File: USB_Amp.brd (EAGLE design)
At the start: 88 x 60 mm, 202 parts, among them CON1 AUDIO_IN, CON2 PROG, CON3 PWR IN, CON4 USB-C-2OZ, CON5 SWD, IC1 ISO7762, IC10 74LVC1G79, IC11 1.8V, IC12 AK1110, IC13 STM32G030F, IC14 CH221, IC15 7808, IC16 TAR5SB33, IC2 3.3V, IC3 PIC32MZEF, IC4 TAR5SB33, IC5 SSM3582, IC6 3G04, IC7 TL431, IC8 74LVC1G79, IC9 74LVC1G79, Q1 PNP, Q2 PNP, Q3 PNP, Q4 NPN, Q5 NPN, X1 12MHz, X2 22.5792MHz, X3 24.576MHz

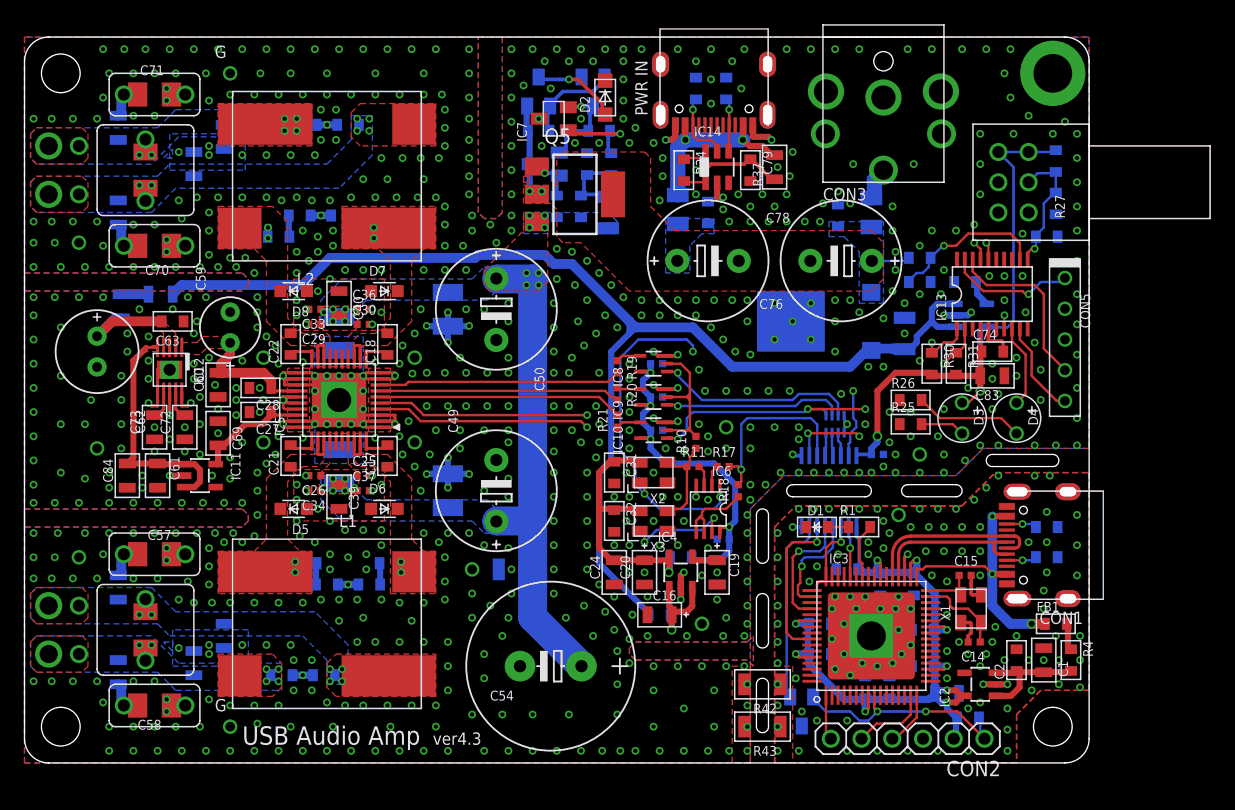
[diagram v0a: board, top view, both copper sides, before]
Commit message: v6
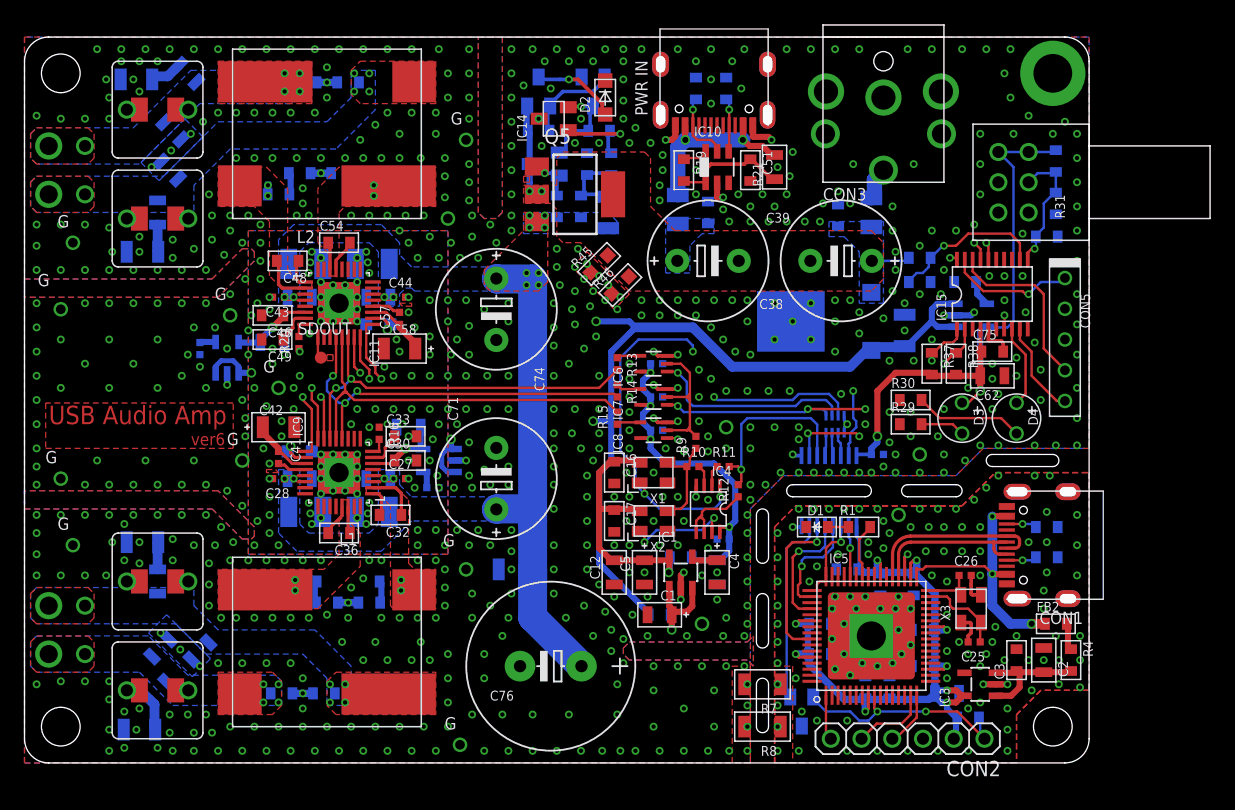
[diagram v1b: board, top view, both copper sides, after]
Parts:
- removed D5, D6, D7, D8: SBD, my_rcl:SOD323
- removed FB6: FB, my_rcl:3216-FB
- added C89: 10n, my_rcl:3216
- added C90, C91: 0.1u, my_rcl:1005
- added IC17: 3.3V, my_ic:SOT23-5
- added R44: 1.5k, my_rcl:1608
- added R45, R46: THJ, my_rcl:1608-W
- added TP23: SDOUT, my_connector:TESTPAD-SMALL
- added TP24: G, my_connector:TESTPIN
- C1, C5: device my_rcl:2012 -> my_rcl:2012-POL
- C12: value 0.1u -> 2.2u; device my_rcl:1608C -> my_rcl:2012
- C13: value 1u -> 0.1u
- C14, C15: value 10p -> 0.1u; device my_rcl:1005 -> my_rcl:1608C
- C16: value 10u -> 0.1u; device my_rcl:2012-POL -> my_rcl:1608C
- C17, C18: value 0.22u -> 0.1u
- C19: value 2.2u -> 0.1u; device my_rcl:2012-POL -> my_rcl:1608C
- C2: value 1u -> 10u; device my_rcl:1608C -> my_rcl:2012
- C20: value 10u -> 0.1u; device my_rcl:2012-POL -> my_rcl:1005
- C21: value 0.22u -> 1u
- C22: value 0.22u -> 0.1u; device my_rcl:1608C -> my_rcl:1005
- C23: value 10u -> 1u; device my_rcl:2012 -> my_rcl:1005
- C24: value 2.2u -> 0.1u; device my_rcl:2012 -> my_rcl:1005
- C25, C26: value 10n -> 10p
- C27, C28, C7: device my_rcl:1608C -> my_rcl:1005
- C29: value 10n -> 1u; device my_rcl:1005 -> my_rcl:2012
- C3: value 0.1u -> 1u
- C30: value 10n -> 1u; device my_rcl:1005 -> my_rcl:1608C
- C31: value 0.1u -> 1u; device my_rcl:1608C -> my_rcl:2012
- C32: value 0.1u -> 0.47u
- C33: value 0.1u -> 1u; device my_rcl:1005 -> my_rcl:1608C
- C34, C35: value 0.1u -> 10u; device my_rcl:1005 -> my_rcl:3225
- C36: value 0.1u -> 0.47u; device my_rcl:1005 -> my_rcl:1608C
- C37: device my_rcl:1005 -> my_rcl:1608C
- C38: value 0.1u -> 25V 1000u; device my_rcl:1005 -> my_rcl:E5-10
- C39: value 1u -> 25V 1000u; device my_rcl:2012 -> my_rcl:E5-10
- C4: value 0.1u -> 2.2u; device my_rcl:1005 -> my_rcl:2012-POL
- C40: device my_rcl:2012 -> my_rcl:1608-W
- C42: value DNP -> 1u; device my_rcl:1608C -> my_rcl:3216-POL
- C43, C44: value 10u -> 0.1u; device my_rcl:3225 -> my_rcl:1005
- C45: value 0.1u -> 1u; device my_rcl:1005 -> my_rcl:2012
- C46: value 10u -> 1u; device my_rcl:3225 -> my_rcl:1608C
- C47: value 10u -> 1u; device my_rcl:3225 -> my_rcl:2012
- C48: value 4.7u -> 0.47u; device my_rcl:3216 -> my_rcl:1608C
- C49: value 16V 680u -> 1u; device my_rcl:E5-10 -> my_rcl:1608C
- C50: value 16V 680u -> 10u; device my_rcl:E5-10 -> my_rcl:3225
- C51: value 100p -> 1u
- C52: value 0.22u -> 10u; device my_rcl:C050W -> my_rcl:3225
- C53: value 100p -> 0.1u
- C54: value 16V 2200u -> 0.47u; device my_rcl:E5-13 -> my_rcl:1608C
- C55: value 1n -> 10u; device my_rcl:2012 -> my_rcl:3216
- C56: value 1n -> 1u; device my_rcl:2012 -> my_rcl:1608-W
- C57: value 10n -> 0.1u; device my_rcl:C050W2 -> my_rcl:1005
- C58: value 10n -> 1u; device my_rcl:C050W2 -> my_rcl:3216-POL
- C59: value 47u -> 0.1u; device my_rcl:E2.5-5 -> my_rcl:1608C
- C60: value 10u -> 100p; device my_rcl:2012 -> my_rcl:1608C
- C61: value 4.7u -> 100p; device my_rcl:2012 -> my_rcl:1608C
- C62: value 100u -> 22u; device my_rcl:E2.5-6.5 -> my_rcl:2012
- C63: value 0.1u -> DNP
- C65: value 0.22u -> 100p; device my_rcl:C050W -> my_rcl:1608C
- C66: value 100p -> 0.47u; device my_rcl:1608C -> my_rcl:C050W
- C67: value 1n -> 0.47u; device my_rcl:2012 -> my_rcl:C050W
- C68: value 1n -> 4.7u; device my_rcl:2012 -> my_rcl:3216
- C69: value 10u -> 1n
- C70: value 10n -> 1n; device my_rcl:C050W2 -> my_rcl:2012
- C71: value 10n -> 16V 680u; device my_rcl:C050W2 -> my_rcl:E5-10
- C72, C73: value 10u -> 10n; device my_rcl:2012 -> my_rcl:3216
- C74: value 0.1u -> 16V 680u; device my_rcl:1608C -> my_rcl:E5-10
- C76: value 25V 1000u -> 16V 2200u; device my_rcl:E5-10 -> my_rcl:E5-13
- C78: value 25V 1000u -> 100p; device my_rcl:E5-10 -> my_rcl:1608C
- C79: value 1u -> 100p
- C8, C9: value 0.1u -> 10u; device my_rcl:1608C -> my_rcl:2012
- C80: value 0.1u -> 100p
- C81: value 10u -> 100p; device my_rcl:3216 -> my_rcl:1608C
- C82: value 0.1u -> 0.47u; device my_rcl:1608C -> my_rcl:C050W
- C83: value 22u -> 0.47u; device my_rcl:2012 -> my_rcl:C050W
- C84: value 4.7u -> 10u
- C85: value 100p -> 10u; device my_rcl:1608C -> my_rcl:2012
- C86, C87: value 100p -> 1n; device my_rcl:1608C -> my_rcl:2012
- C88: value 100p -> 10n; device my_rcl:1608C -> my_rcl:3216
- FB4: device my_rcl:2012-R -> my_rcl:3216-FB
- IC1: value ISO7762 -> TAR5SB33; device my_ic:TSSOP16 -> my_ic:SOT23-5
- IC10: value 74LVC1G79 -> CH221; device my_ic:TSSOP5 -> my_ic:SOT23-6
- IC11: value 1.8V -> TAS5827; device my_ic:SOT23-5 -> my_ic:QFN32-TAS
- IC12: value AK1110 -> 7805; device my_ic:PLP10 -> my_ic:DPAK
- IC13: value STM32G030F -> TAR5SB33; device my_ic:TSSOP20 -> my_ic:SOT23-5
- IC14: value CH221 -> TL431; device my_ic:SOT23-6 -> my_ic:SC59
- IC15: value 7808 -> STM32G030F; device my_ic:DPAK -> my_ic:TSSOP20
- IC16: value TAR5SB33 -> 3.3V
- IC2: value 3.3V -> ISO7762; device my_ic:SOT23-5 -> my_ic:TSSOP16
- IC3: value PIC32MZEF -> 3.3V; device my_ic:QFN64HT -> my_ic:SOT23-5
- IC4: value TAR5SB33 -> 3G04; device my_ic:SOT23-5 -> my_ic:SSOP8-P-0.65
- IC5: value SSM3582 -> PIC32MZEF; device my_ic:QFN40HT -> my_ic:QFN64HT
- IC6: value 3G04 -> 74LVC1G79; device my_ic:SSOP8-P-0.65 -> my_ic:TSSOP5
- IC7: value TL431 -> 74LVC1G79; device my_ic:SC59 -> my_ic:TSSOP5
- IC9: value 74LVC1G79 -> TAS5827; device my_ic:TSSOP5 -> my_ic:QFN32-TAS
- R11: value 51 -> MCLK
- R12: value 39.2k -> MCLKB; device my_rcl:1608 -> my_rcl:1005
- R13: value 10k -> DATA; device my_rcl:1608 -> my_rcl:1005
- R14: value 1k -> LRCLK; device my_rcl:3216 -> my_rcl:1005
- R15: value 51 -> SCK; device my_rcl:2012 -> my_rcl:1005
- R16: value 51 -> 0; device my_rcl:2012 -> my_rcl:1005
- R17: value MCLK -> 5.1k; device my_rcl:1005 -> my_rcl:1608
- R18: value MCLKB -> 5.1k; device my_rcl:1005 -> my_rcl:1608
- R19: value SCK -> 200k; device my_rcl:1005 -> my_rcl:1608
- R20: value DATA -> 1k
- R21: value LRCLK -> 1k; device my_rcl:1005 -> my_rcl:2012
- R22: value 2.2 -> 100; device my_rcl:2012-R -> my_rcl:1608
- R23, R24: value 51 -> 10; device my_rcl:2012 -> my_rcl:1608
- R25, R26: value 3.3k -> 1k
- R27: value 50k -> 40.2k; device my_rcl:RK0972 -> my_rcl:1608
- R28: value DNP -> 10k
- R29: value 100k -> 3.3k
- R30: value 10k -> 3.3k
- R31: value 10k -> 50k; device my_rcl:1608 -> my_rcl:RK0972
- R32, R33: value 5.1k -> 5.1; device my_rcl:1608 -> my_rcl:2012
- R34: value 100k -> 1k; device my_rcl:1608 -> my_rcl:3216
- R35: value 10k -> DNP
- R36: value 1.5k -> 100k
- R37: value 1k -> 10k; device my_rcl:2012 -> my_rcl:1608
- R38: value 10 -> 10k
- R41: value 10 -> 5.1; device my_rcl:1608 -> my_rcl:2012
- R42: value THJ -> 5.1; device my_rcl:3216-2 -> my_rcl:2012
- R43: value THJ -> 10k; device my_rcl:3216-2 -> my_rcl:1608
- R7: value 100 -> THJ; device my_rcl:1608 -> my_rcl:3216-2
- R8: value 1k -> THJ; device my_rcl:1608 -> my_rcl:3216-2
- R9: value 1k -> 51; device my_rcl:1608 -> my_rcl:1005
- TP19: value L_P -> L_N
- TP22, TP4: value R_N -> R_P
- TP3: value R_P -> R_N
- X1: value 12MHz -> 22.5792MHz; device my_rcl:KC3225-CRYSTAL -> my_rcl:KC3225
- X2: value 22.5792MHz -> 24.576MHz
- X3: value 24.576MHz -> 12MHz; device my_rcl:KC3225 -> my_rcl:KC3225-CRYSTAL
- moved C62 74.0 mm to (80.0, 32.0), turned to 0 degrees
- moved C83 72.4 mm to (11.0, 54.0), turned to 180 degrees
- moved R42 69.3 mm to (13.5, 57.0), flipped to the bottom, turned to 225 degrees
- moved C82 67.0 mm to (11.0, 45.0), flipped to the top
- moved R33 66.7 mm to (11.0, 6.00), turned to 135 degrees
- moved R32 62.2 mm to (11.0, 15.0)
- moved C55 61.7 mm to (72.8, 35.8)
- moved C59 60.9 mm to (77.8, 39.8), flipped to the bottom, turned to 0 degrees
- moved FB4 59.1 mm to (70.0, 45.5), turned to 270 degrees
- moved IC12 58.1 mm to (70.0, 36.5), flipped to the bottom, turned to 270 degrees
- moved R38 56.2 mm to (77.0, 33.0), flipped to the top, turned to 270 degrees
- moved C51 54.6 mm to (60.0, 49.0), flipped to the top, turned to 270 degrees
- moved C26 54.4 mm to (77.8, 15.5), turned to 0 degrees
- moved C81 53.7 mm to (23.2, 56.2), turned to 180 degrees
- moved C21 53.1 mm to (71.5, 6.25), flipped to the bottom
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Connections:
- removed net +8V: C81.1, FB2.1, FB4.1, IC15.3, IC16.1, IC16.3
- removed net AMP_+5V: C61.1, C84.1, IC11.1, IC11.3, IC12.5
- removed net AMP_AVDD: C28.1, C59.+, C60.1, IC12.1, IC5.24
- removed net AMP_DVDD: C27.1, C69.1, IC11.5, IC5.28
- new net +5V: C55.1, FB1.1, IC12.3, IC13.1, IC13.3, IC16.1, IC16.3, IC17.1, IC17.3
- new net AMP_AVDD_L: C41.1, C42.1, IC9.19
- new net AMP_AVDD_R: C57.1, C58.1, IC11.19
- new net AMP_DVDD_L: C30.1, C84.1, IC16.5, IC9.6
- new net AMP_DVDD_R: C46.1, C85.1, IC11.6, IC17.5
- new net AMP_EN: IC11.17, IC15.20, IC9.17
- new net AMP_IO0: IC11.9, TP23.1
- new net N$47: IC11.8, R20.2
- new net N$48: C33.1, IC9.7
- new net N$49: C90.1, IC16.4
- new net N$50: C91.1, IC17.4
- net +12V: now also C27.1, C28.1, C31.1, C35.1, C45.1, C50.1, C52.1, C68.1, C71.+, C74.+, C76.+, IC11.21, IC11.22, IC11.3, IC11.4, IC9.21, IC9.22, IC9.3, IC9.4, R25.2, R27.2, R34.2; no longer C25.1, C26.1, C30.1, C33.1, C36.1, C37.1, C39.1, C40.1, C46.1, C48.1, C49.+, C50.+, C54.+, IC5.14, IC5.15, IC5.16, IC5.17, IC5.34, IC5.35, IC5.36, IC5.37, R12.2, R14.2, R8.2
- net +3V3: now also C62.1, C7.1, C75.1, IC13.5, IC15.4, IC2.16, R31.3, R31.6, R35.2, R37.2, R38.2; no longer C4.1, C74.1, C83.1, IC1.16, IC13.4, IC16.5, R27.3, R27.6, R28.2, R30.2, R31.2
- net +3V3A: now also C20.1, C22.1, C24.1, C8.1, IC4.8, IC6.5, IC7.5; no longer C35.1, C38.1, C41.1, C45.1, IC10.5, IC6.8, IC9.5
- net +3V3D: now also C14.1, C15.1, C18.1, C19.1, C21.1, IC2.1, IC3.5, IC5.19, IC5.26, IC5.34, IC5.39, IC5.54, IC5.60, IC5.8; no longer C12.1, C3.1, C5.1, C7.1, C8.1, IC1.1, IC2.5, IC3.19, IC3.26, IC3.34, IC3.39, IC3.54, IC3.60, IC3.8
- net AMP_OUTN_L: now also C36.1, IC9.30, R24.2; no longer C21.1, D5.2, IC5.32, IC5.33, R38.2
- net AMP_OUTN_R: now also C54.1, IC11.30, L2.1, R39.2; no longer C22.2, D8.2, IC5.18, IC5.19, L2.4, R40.2
- net AMP_OUTP_L: now also C32.1, IC9.2, R23.2; no longer C17.1, D6.2, IC5.38, IC5.39, R39.2
- net AMP_OUTP_R: now also C48.2, IC11.2, L2.4, R40.2; no longer C18.2, D7.2, IC5.12, IC5.13, L2.1, R41.2
- net DGND: now also C18.2, C19.2, C21.2, C25.2, C26.2, IC2.8, IC3.2, IC5.20, IC5.25, IC5.35, IC5.40, IC5.55, IC5.59, IC5.7, IC5.HT, IC5.HT2, R7.1, R8.1, X3.2, X3.4; no longer C1.2, C12.2, C5.2, C7.2, C8.2, IC1.8, IC2.2, IC3.20, IC3.25, IC3.35, IC3.40, IC3.55, IC3.59, IC3.7, IC3.HT, IC3.HT2, R42.1, R43.1, X1.2, X1.4
- net EN_441K: now also IC15.17, IC2.15, IC4.1, X1.1; no longer IC1.15, IC13.17, IC6.1, X2.1
- net EN_48K: now also IC4.7, X2.1; no longer IC6.7, X3.1
- net GND: now also C1.2, C12.2, C17.2, C22.2, C38.-, C39.-, C42.2, C49.2, C5.2, C50.2, C51.2, C52.2, C55.2, C57.2, C59.2, C62.2, C65.2, C66.1, C66.3, C67.2, C67.4, C69.1, C7.2, C70.2, C71.-, C72.1, C74.-, C78.2, C8.2, C80.1, C82.1, C82.3, C83.4, C86.1, C88.1, C89.2, C90.2, C91.2, IC1.2, IC10.2, IC11.20, IC11.25, IC11.26, IC11.31, IC11.32, IC11.5, IC11.HT, IC11.HT2, IC12.2, IC13.2, IC14.3, IC15.5, IC17.2, IC2.9, IC4.4, IC6.3, IC9.20, IC9.25, IC9.26, IC9.31, IC9.32, IC9.5, IC9.HT, IC9.HT2, R16.1, R17.2, R18.2, R20.1, R28.1, R30.1, R31.1, R31.4, R34.1, R36.1, R44.2, R45.1, R46.1, R7.2, R8.2, TP24.1, X1.2; no longer C19.2, C25.2, C26.2, C32.2, C36.2, C38.2, C39.2, C49.-, C50.-, C51.1, C54.-, C55.1, C57.1, C57.3, C58.4, C59.-, C62.-, C63.2, C66.2, C67.1, C68.2, C69.2, C70.1, C70.3, C71.2, C71.4, C72.2, C74.2, C78.-, C80.2, C82.2, C86.2, C88.2, D5.1, D6.1, D7.1, D8.1, IC1.9, IC10.3, IC11.2, IC12.10, IC12.6, IC12.8, IC12.HT, IC12.HT2, IC13.5, IC14.2, IC15.2, IC4.2, IC5.1, IC5.10, IC5.2, IC5.21, IC5.22, IC5.23, IC5.25, IC5.26, IC5.27, IC5.29, IC5.3, IC5.30, IC5.9, IC5.HT, IC5.HT2, IC6.4, IC9.3, R13.1, R14.1, R25.1, R26.1, R27.1, R27.4, R32.2, R33.2, R36.2, R42.2, R43.2, X3.2
- net I2C_SCL: now also IC11.16, IC15.1, IC9.16, R37.1; no longer IC13.1, IC5.4, R30.1
- net I2C_SDA: now also IC11.15, IC15.2, IC9.15, R38.1; no longer IC13.2, IC5.5, R31.1
- net I2S_DATA: now also IC6.1; no longer IC9.1
- net I2S_DATA_BUF: now also IC11.14, IC9.14, R13.2; no longer IC5.7, R20.2
- net I2S_LRCLK: now also IC15.7, IC7.1; no longer IC10.1, IC13.7
- net I2S_LRCLK_BUF: now also IC11.12, IC9.12, R14.2; no longer IC5.6, R21.2
- net I2S_MCLK: now also IC6.2, IC7.2, R9.2; no longer IC10.2, IC9.2, R10.2
- net I2S_MCLK2: now also IC4.3, R10.2; no longer IC6.3, R11.2
- net I2S_MCLK_BUF: now also IC2.11, R11.2, R12.2; no longer IC1.11, R17.2, R18.2
- net I2S_SCK_BUF: now also IC11.13, IC9.13, R15.2; no longer IC5.8, R19.2
- net LED0: now also IC15.8; no longer IC13.8
- net LED1: now also IC5.42; no longer IC3.42
- net MCLK_OSC: now also R9.1, X1.3; no longer R11.1, X3.3
- net MCLR: now also IC5.9; no longer IC3.9
- net N$10: now also IC6.4, R13.1; no longer IC8.4, R19.1
- net N$11: now also IC7.4, R14.1; no longer IC9.4, R20.1
- net N$12: now also C54.2, IC11.29; no longer C21.2, IC5.31
- net N$13: now also C32.2, IC9.1; no longer C17.2, IC5.40
- net N$14: now also IC8.4, R15.1; no longer IC10.4, R21.1
- net N$15: now also C73.1, R33.1; no longer C58.1, C58.3, R16.1
- net N$16: now also R25.1; no longer R8.1
- net N$17: now also C40.1, IC9.18; no longer C18.1, IC5.11
- net N$18: now also C36.2, IC9.29; no longer C22.1, IC5.20
- net N$19: now also C89.1, R42.1; no longer C71.1, C71.3, R24.1
- net N$20: now also C63.2, IC14.1, R26.1; no longer C42.2, IC7.1, R9.1
- net N$21: now also C88.2, R41.2; no longer C70.2, C70.4, R23.2
- net N$22: now also IC2.13; no longer IC1.13
- net N$23: now also C4.1, IC1.4; no longer C19.1, IC4.4
- net N$24: now also IC2.12; no longer IC1.12
- net N$25: now also C63.1, IC14.2; no longer C42.1, IC7.2
- net N$26: now also IC9.8, R16.2; no longer C73.1, IC12.7
- net N$27: now also C56.1, IC11.18; no longer C72.1, IC12.9
- net N$28: now also R22.1; no longer R7.1
- net N$29: now also C48.1, IC11.1; no longer C62.+, C63.1, IC12.2, IC12.3, IC12.4, R22.2
- net N$3: now also FB2.2; no longer FB1.2
- net N$30: now also C68.2, R26.2, R27.1, R28.2; no longer C48.2, R12.1, R13.2, R9.2
- net N$31: now also IC10.4, R17.1; no longer IC14.4, R32.1
- net N$32: now also IC10.5, R18.1; no longer IC14.5, R33.1
- net N$33: now also C51.1, IC10.1, R19.2, R21.1; no longer C79.1, IC14.1, R34.2, R37.1
- net N$34: now also IC10.6, R19.1; no longer IC14.6, R34.1
- net N$35: now also C59.1, IC13.4; no longer C82.1, IC16.4
- net N$36: now also R29.2; no longer R25.2
- net N$37: now also IC4.5, IC4.6, R12.1; no longer IC6.5, IC6.6, R18.1
- net N$39: now also IC4.2, R11.1; no longer IC6.2, R17.1
- net N$4: now also C3.1, IC3.1, IC3.3; no longer C1.1, IC2.1, IC2.3
- net N$40: now also C60.1, R23.1; no longer C86.1, R39.1
- net N$41: now also R30.2; no longer R26.2
- net N$42: now also C49.1, IC11.7; no longer FB4.2, R22.1
- net N$43: now also C1.1, FB1.2, IC1.1, IC1.3; no longer C16.1, FB2.2, IC4.1, IC4.3
- net N$44: now also C79.1; no longer C87.1
- net N$45: now also C61.1, R24.1; no longer C85.1, R38.1
- net N$46: now also C78.1, R39.1; no longer C88.1, R41.1
- net N$5: now also C25.1, IC5.31, X3.3; no longer C14.1, IC3.31, X1.3
- net N$6: now also C72.2, R32.2; no longer C57.2, C57.4, R15.2
- net N$7: now also C26.1, IC5.32, X3.1; no longer C15.1, IC3.32, X1.1
- net N$8: now also IC2.14; no longer IC1.14
- net PGEC: now also IC5.15; no longer IC3.15
- net PGED: now also IC5.16; no longer IC3.16
- net PIC_DATA: now also IC2.4, IC5.50; no longer IC1.4, IC3.50
- net PIC_DDC_EN: now also IC2.7; no longer IC1.7
- net PIC_EN441K: now also IC2.2, IC5.44; no longer IC1.2, IC3.44
- net PIC_LRCLK: now also IC2.5, IC5.52; no longer IC1.5, IC3.52
- net PIC_MCLK: now also IC2.6, IC5.57; no longer IC1.6, IC3.57
- net PIC_SCK: now also IC2.3, IC5.48, IC5.49; no longer IC1.3, IC3.48, IC3.49
- net SPK_OUTN_L: now also C65.1, C67.1, C67.3, C70.1, R33.2; no longer C52.2, C52.4, C53.1, C56.1, R16.2
- net SPK_OUTN_R: now also C80.2, C82.2, C82.4, C86.2, L2.2, R41.1, TP21.1, TP3.1; no longer C65.2, C65.4, C66.1, C68.1, L2.3, R24.2, TP22.1, TP4.1
- net SPK_OUTP_L: now also C64.2, C66.2, C66.4, C69.2, R32.1; no longer C51.2, C52.1, C52.3, C55.2, R15.1
- net SPK_OUTP_R: now also C81.1, C83.1, C83.3, C87.1, L2.3, R42.2, TP22.1, TP4.1; no longer C64.2, C65.1, C65.3, C67.2, L2.2, R23.1, TP21.1, TP3.1
- net STM_DDC_EN: now also IC15.16, IC2.10; no longer IC1.10, IC13.16
- net STM_TX: now also IC15.9; no longer IC13.9
- net SWCLK: now also IC15.19; no longer IC13.19
- net SWDIO: now also IC15.18; no longer IC13.18
- net UART_TX: now also IC5.1; no longer IC3.1
- net USB_D+: now also IC5.37; no longer IC3.37
- net USB_D-: now also IC5.36; no longer IC3.36
- net USB_VBUS: now also FB2.1, IC5.33; no longer FB1.1, IC3.33
- net V+: now also C37.1, C38.+, C39.+, C53.1, FB4.2, IC12.1, R22.2, R43.2, R45.2, R46.2; no longer C75.1, C76.+, C78.+, C80.1, FB6.2, IC15.1, R35.2, R7.2
- net V+_ADC: now also IC15.12, R43.1, R44.1; no longer IC13.12, R35.1, R36.1
- net VIN+: now also FB4.1; no longer FB5.1
- net VINC_+: now also FB5.1, R21.2; no longer FB6.1, R37.2
- net VOL_ADC: now also IC15.11, R31.2, R31.5, R35.1, R36.2; no longer IC13.11, R27.2, R27.5, R28.1, R29.2
- net XVCC: now also C12.1, C16.1, C17.1, C5.1, IC1.5, X1.4; no longer C20.1, C24.1, C31.1, C32.1, IC4.5, X3.4
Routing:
- net +5V: track 0.00 -> 117.5 mm, vias 0 -> 4
- net +8V: track 102.8 -> 0.00 mm
- net AMP_EN: track 0.00 -> 80.9 mm, vias 0 -> 3
- net GND: track 95.0 -> 41.6 mm, vias 791 -> 776
- net AMP_+5V: track 19.9 -> 0.00 mm
- net I2S_LRCLK_BUF: track 20.2 -> 32.8 mm, vias 0 -> 3
- net I2S_DATA_BUF: track 19.9 -> 32.5 mm, vias 0 -> 2
- net I2S_SCK_BUF: track 20.0 -> 32.5 mm
- net I2C_SDA: track 57.8 -> 69.3 mm, vias 2 -> 3
- net AMP_AVDD: track 10.6 -> 0.00 mm
- net AMP_DVDD: track 9.74 -> 0.00 mm
- net I2C_SCL: track 61.2 -> 70.6 mm, vias 2 -> 3
- net AMP_DVDD_R: track 0.00 -> 6.86 mm, vias 0 -> 1
- net AMP_DVDD_L: track 0.00 -> 6.55 mm, vias 0 -> 1
- net N$29: track 8.47 -> 2.37 mm
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- removed copper zone on layer 1, net AMP_+5V
- removed copper zone on layer 1, net AMP_AVDD
- removed copper zone on layer 1, net GND1
- removed copper zone on layer 15, net GND1
- removed copper zone on layer 16, net GND1
- removed copper zone on layer 2, net GND2
- removed copper zone on layer 1, net GND3
- removed copper zone on layer 15, net GND3
- removed copper zone on layer 16, net GND3
- removed copper zone on layer 1, net N$29
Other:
- board text added: "ver6"
- board text removed: "ver4.3"
